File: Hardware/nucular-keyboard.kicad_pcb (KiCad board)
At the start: 2 copper layers, 48 x 25 mm, 34 parts, among them IC1 STM32L052R6Tx, J1 JAE_AA01B-S040VA1, J2 JAE_KX14-40K2D, J3 CONN_01X16, J4 CONN_01X03, Q1 IRLML6402, U1 MCP1700T-3302E/MB

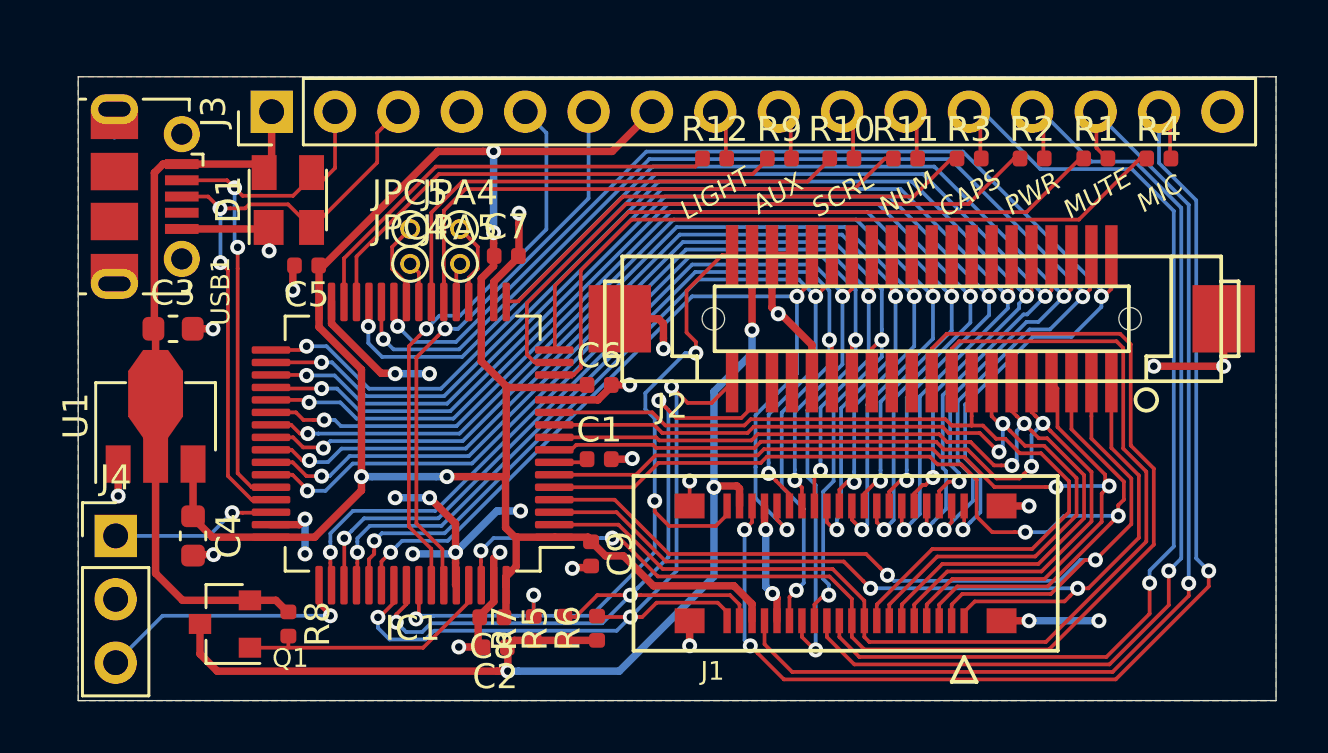
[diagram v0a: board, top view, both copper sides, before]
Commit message: Finished routing
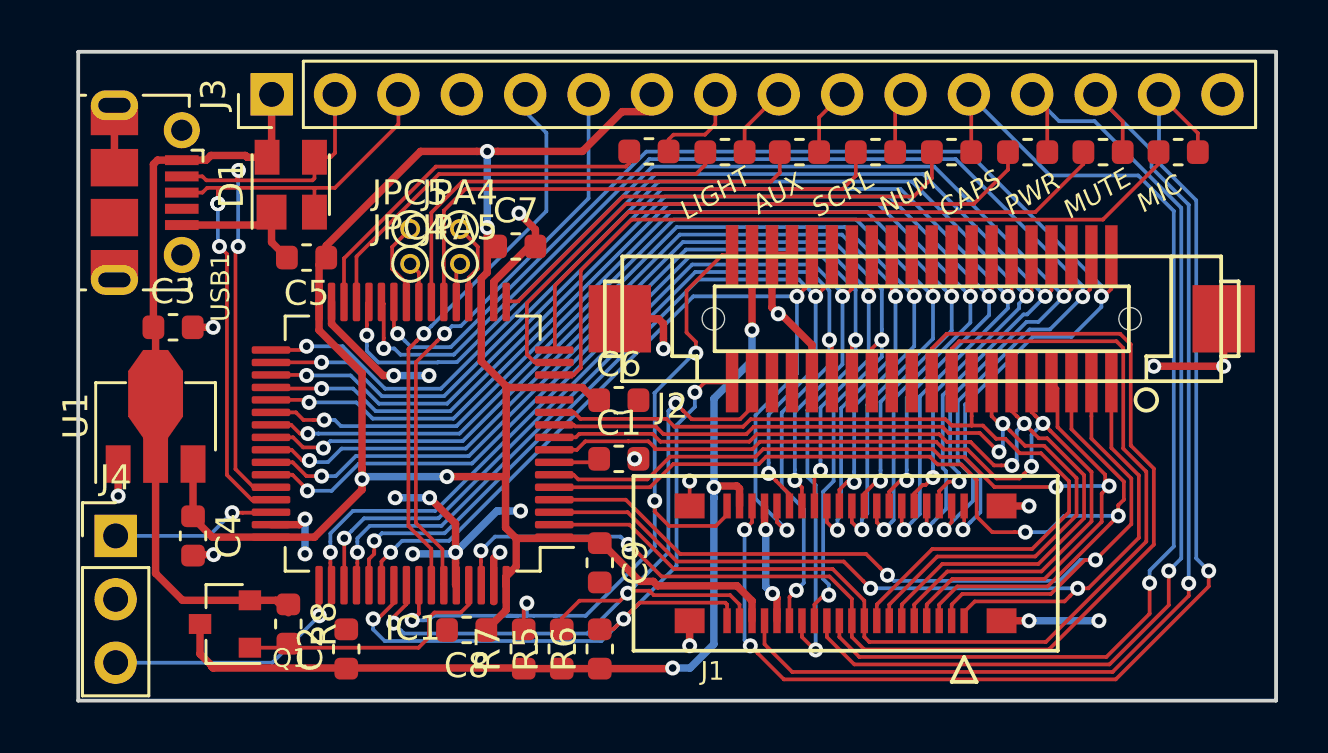
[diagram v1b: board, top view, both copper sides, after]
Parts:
- C1, C2, C5, C6, C7, C8, C9: footprint Capacitor_SMD:C_0402_1005Metric -> Capacitor_SMD:C_0603_1608Metric
- R1, R10, R11, R12, R2, R3, R4, R5, R6, R7, R8, R9: footprint Resistor_SMD:R_0402_1005Metric -> Resistor_SMD:R_0603_1608Metric
- moved C2 5.97 mm to (70.7, 82.9), turned to 90 degrees
- moved R12 2.65 mm to (82.9, 63.0)
- moved R9 2.20 mm to (85.9, 63.0)
- moved R10 1.72 mm to (88.9, 63.0)
- moved R11 1.23 mm to (91.9, 63.0)
- moved C8 1.13 mm to (75.6, 82.2)
- moved C6 1.00 mm to (81.7, 73.0)
- moved R7 0.91 mm to (77.9, 82.9)
- moved R6 0.84 mm to (80.9, 82.9)
- moved R5 0.84 mm to (79.4, 82.9)
- moved R4 0.82 mm to (104.1, 63.0)
- moved C1 0.79 mm to (81.7, 75.3)
- moved R3 0.75 mm to (95.0, 63.0)
- moved J3 0.69 mm to (67.8, 60.7)
- moved D1 0.63 mm to (68.5, 64.3)
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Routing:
- net GND: track 67.9 -> 62.5 mm, vias 31 -> 26
- net /+5V_TP: track 43.6 -> 40.5 mm
- net /LED_LIGHT: track 17.8 -> 15.2 mm
- net /LED_AUX: track 19.9 -> 17.8 mm
- net VCC: track 75.9 -> 77.7 mm
- net /LED_LIGHT_R: track 2.02 -> 3.80 mm
- net /LED_MIC_R: track 48.3 -> 49.8 mm
- net /USB_DM: track 22.2 -> 23.7 mm
- net /LED_SCROLL: track 20.5 -> 19.0 mm
- net /LED_MUTE_R: track 42.7 -> 44.1 mm
- net /TP4_PWR: track 10.7 -> 11.9 mm
- net Net-(IC1-Pad20): track 3.37 -> 4.34 mm
- net /LED_NUM: track 22.6 -> 21.7 mm
- net /LED_MIC: track 29.7 -> 30.5 mm
- net /LED_AUX_R: track 2.07 -> 2.88 mm
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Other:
- board size 48 x 25 mm -> 48 x 26 mm

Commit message: Moved references
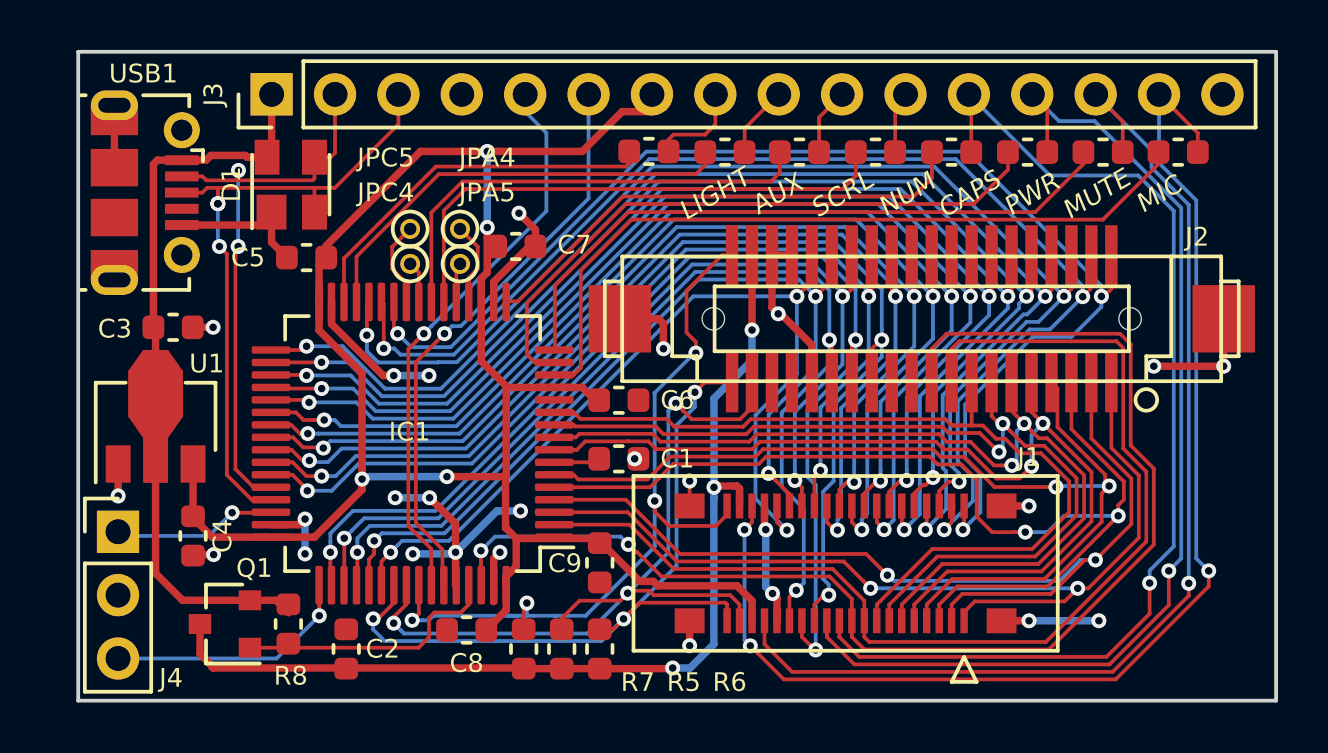
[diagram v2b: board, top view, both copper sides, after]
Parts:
- moved J4 0.19 mm to (61.6, 78.2)
